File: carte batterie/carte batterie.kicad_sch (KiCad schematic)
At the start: 11 parts, among them IC1 TPS3711DDCT, J1 Conn_01x02_Pin, J2 Conn_01x02_Pin, J3 Conn_01x01_Pin, Q1 SI3127DV-T1-GE3, U1 ATtiny1616-S

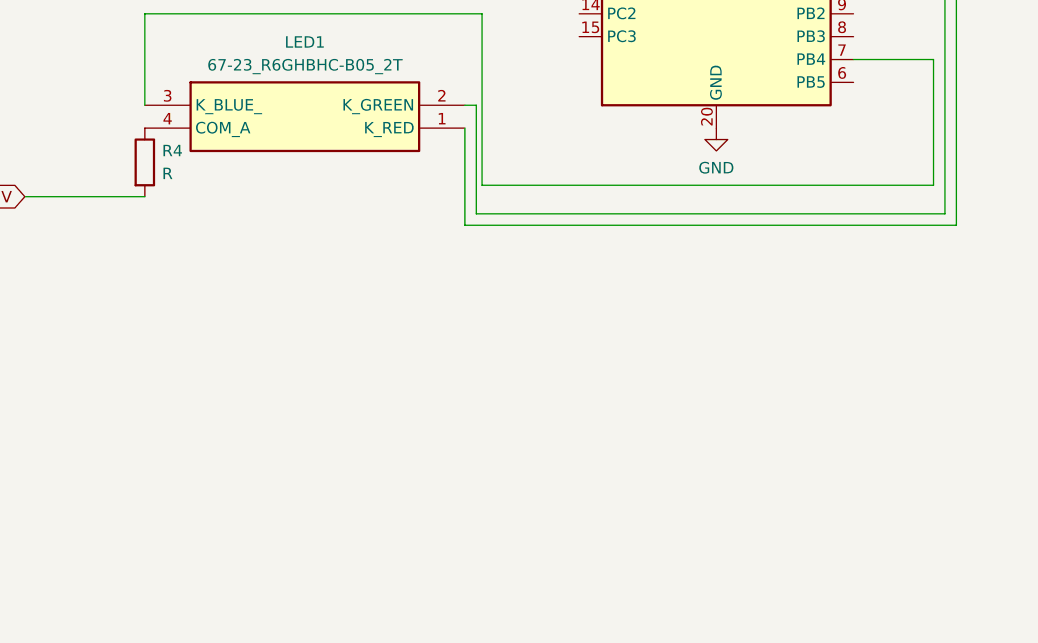
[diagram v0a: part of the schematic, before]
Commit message: new compo
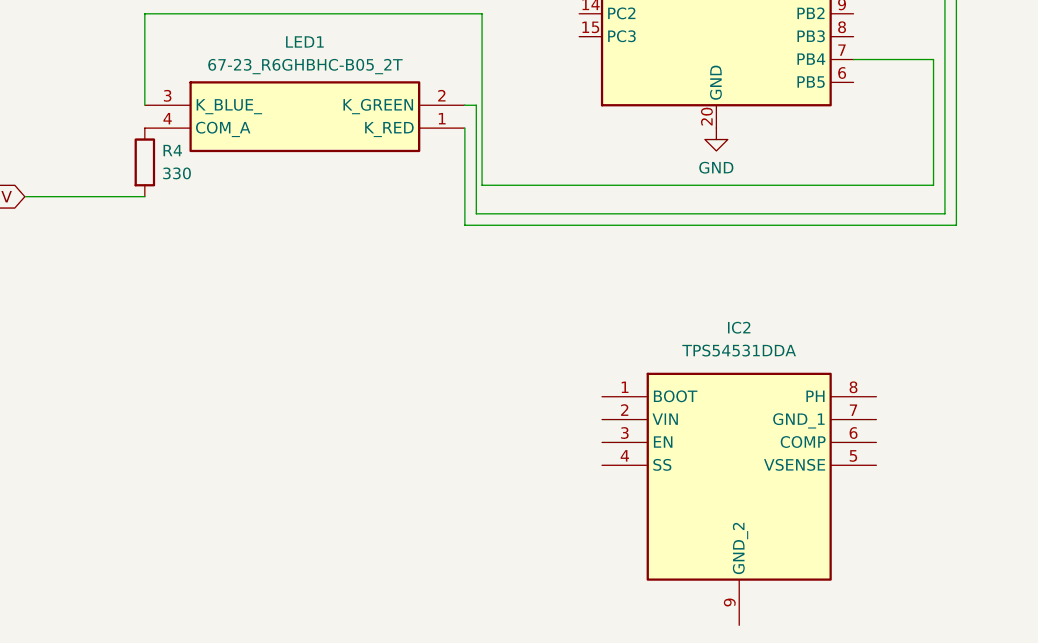
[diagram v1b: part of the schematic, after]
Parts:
- added IC2: TPS54531DDA, SOIC127P600X170-9N, symbol SamacSys_Parts:TPS54531DDA
- R4: value R -> 330
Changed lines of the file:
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@@
       (effects (font (size 1.27 1.27)) (justify left))
     )
-    (property "Value" "R" (at 54.61 104.775 0)
+    (property "Value" "330" (at 54.61 104.775 0)
       (effects (font (size 1.27 1.27)) (justify left))
     )
@@
         )
       )
+    )
+  )
+  (symbol (lib_id "SamacSys_Parts:TPS54531DDA") (at 103.505 129.54 0) (unit 1)
+    (in_bom yes) (on_board yes) (dnp no) (fields_autoplaced)
+    (property "Reference" "IC2" (at 118.745 121.92 0)
+      (effects (font (size 1.27 1.27)))
+    )
+    (property "Value" "TPS54531DDA" (at 118.745 124.46 0)
+      (effects (font (size 1.27 1.27)))
+    )
+    (property "Footprint" "SOIC127P600X170-9N" (at 130.175 224.46 0)
+      (effects (font (size 1.27 1.27)) (justify left top) hide)
+    )
+    (property "Datasheet" "http://www.ti.com/lit/gpn/tps54531" (at 130.175 324.46 0)
+      (effects (font (size 1.27 1.27)) (justify left top) hide)
+    )
+    (property "Height" "1.7" (at 130.175 524.46 0)
+      (effects (font (size 1.27 1.27)) (justify left top) hide)
+    )
+    (property "Manufacturer_Name" "Texas Instruments" (at 130.175 624.46 0)
+      (effects (font (size 1.27 1.27)) (justify left top) hide)
+    )
+    (property "Manufacturer_Part_Number" "TPS54531DDA" (at 130.175 724.46 0)
+      (effects (font (size 1.27 1.27)) (justify left top) hide)
+    )
+    (property "Mouser Part Number" "595-TPS54531DDA" (at 130.175 824.46 0)
+      (effects (font (size 1.27 1.27)) (justify left top) hide)
+    )
+    (property "Mouser Price/Stock" "https://www.mouser.co.uk/ProductDetail/Texas-Instruments/TPS54531DDA?qs=jA5Ki6243omoJVKISZs%2FBg%3D%3D" (at 130.175 924.46 0)
+      (effects (font (size 1.27 1.27)) (justify left top) hide)
+    )
+    (property "Arrow Part Number" "TPS54531DDA" (at 130.175 1024.46 0)
+      (effects (font (size 1.27 1.27)) (justify left top) hide)
+    )
+    (property "Arrow Price/Stock" "https://www.arrow.com/en/products/tps54531dda/texas-instruments?region=nac" (at 130.175 1124.46 0)
+      (effects (font (size 1.27 1.27)) (justify left top) hide)
+    )
+    (pin "1")
+    (pin "2")
+    (pin "3")
+    (pin "4")
+    (pin "5")
+    (pin "6")
+    (pin "7")
+    (pin "8")
+    (pin "9")
+    (instances
+      (project "carte batterie"
+        (path "/8afff8df-3578-4f51-814d-4ef430aba141"
+          (reference "IC2") (unit 1)
+        )
+      )
